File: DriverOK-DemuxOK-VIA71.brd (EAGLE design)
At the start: 129.8 x 170.2 mm, 55 parts, among them X1 1613_14

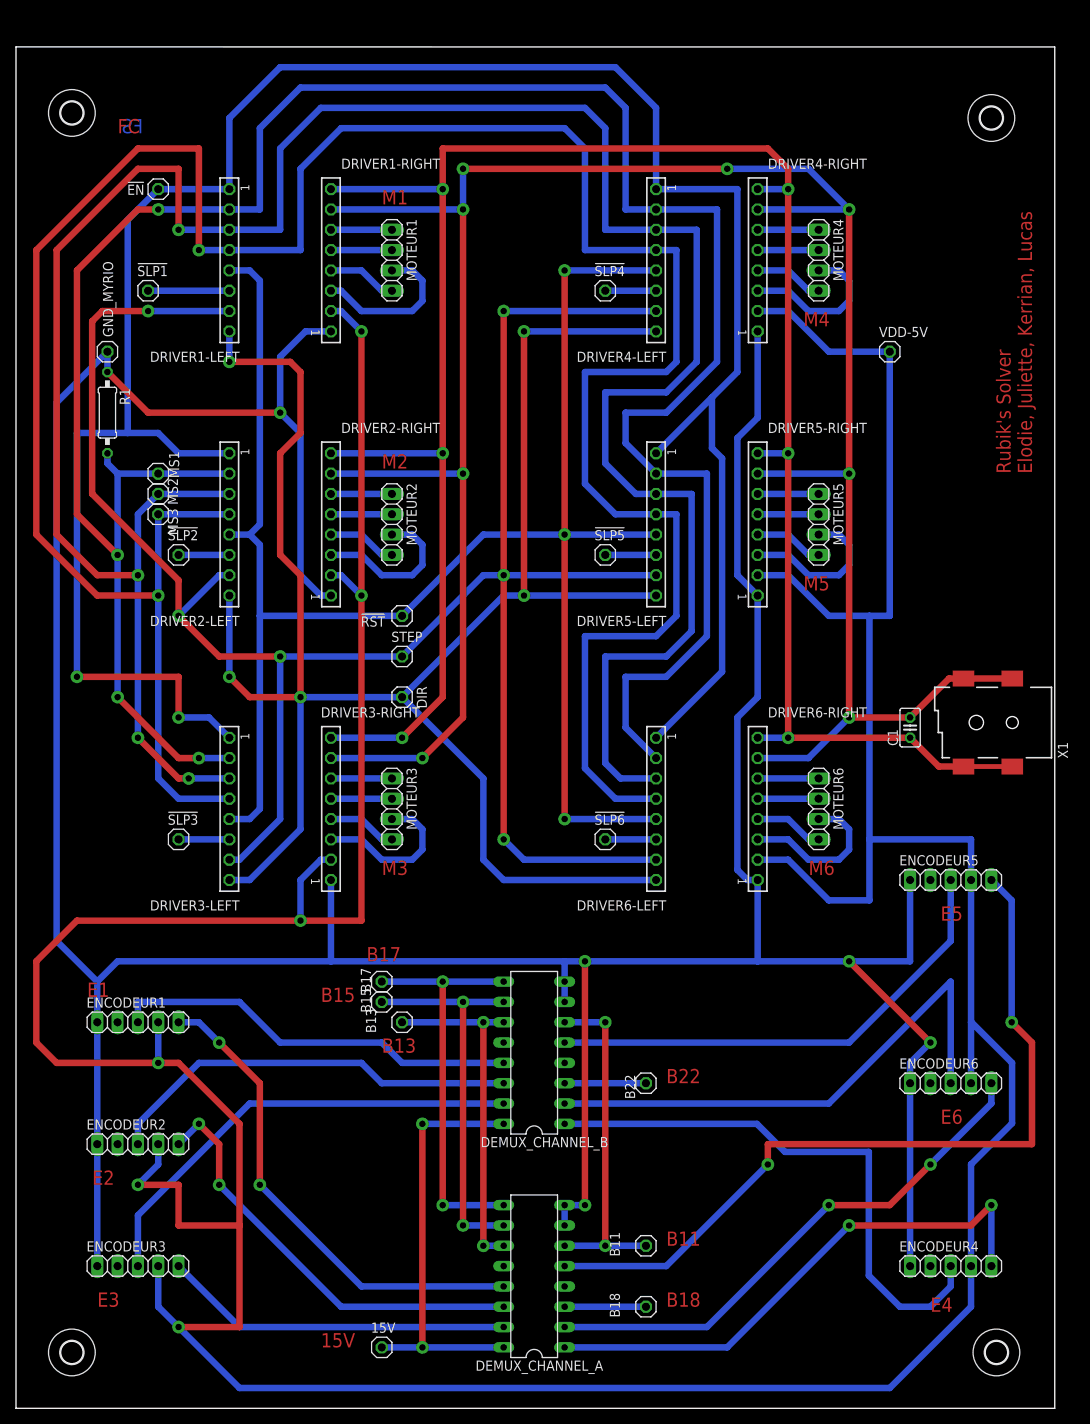
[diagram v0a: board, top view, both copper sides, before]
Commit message: Update largeur de la board
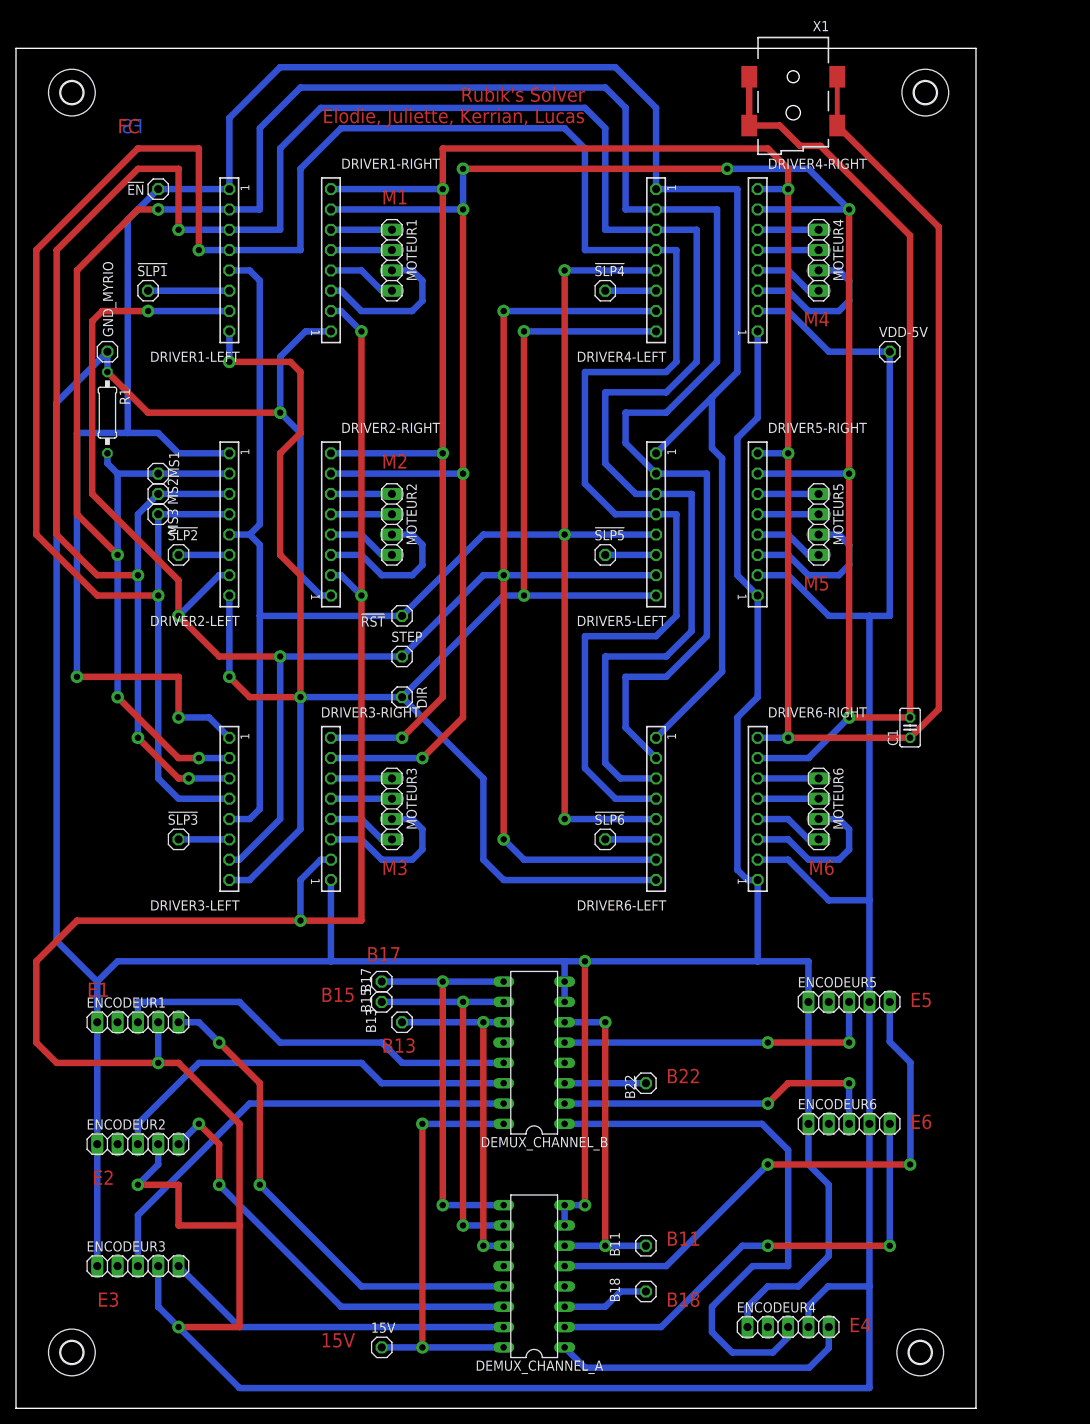
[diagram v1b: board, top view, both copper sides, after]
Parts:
- moved X1 91.6 mm to (97.2, 171.4), turned to 180 degrees
- moved ENCODEUR4 21.7 mm to (96.5, 10.2)
- moved ENCODEUR5 19.8 mm to (104.1, 50.8)
- moved ENCODEUR6 13.7 mm to (104.1, 35.6)
- moved H4 9.53 mm to (113.0, 6.99)
- moved H3 8.84 mm to (113.7, 164.5)
- moved H1 2.54 mm to (6.99, 164.5)
- moved B18 1.91 mm to (78.7, 14.6)
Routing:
- net GND_ALIM: track 292.9 -> 370.2 mm
- net 24V: track 268.9 -> 344.0 mm
- net E5-A: track 101.3 -> 69.9 mm
- net E4-A: track 68.3 -> 37.7 mm, vias 2 -> 0
- net 5V: track 557.9 -> 530.1 mm
- net E6-B: track 67.3 -> 41.7 mm, vias 0 -> 2
- net E5-B: track 61.1 -> 40.6 mm, vias 0 -> 2
- net GND_MYRIO: track 476.8 -> 463.8 mm, vias 5 -> 3
- net E6-A: track 67.5 -> 60.1 mm
- net E4-B: track 70.4 -> 71.2 mm
- net B18: track 10.2 -> 10.9 mm
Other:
- board size 129.8 x 170.2 mm -> 120 x 170 mm
